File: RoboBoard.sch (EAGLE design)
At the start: 23 parts, among them IC2 L293D

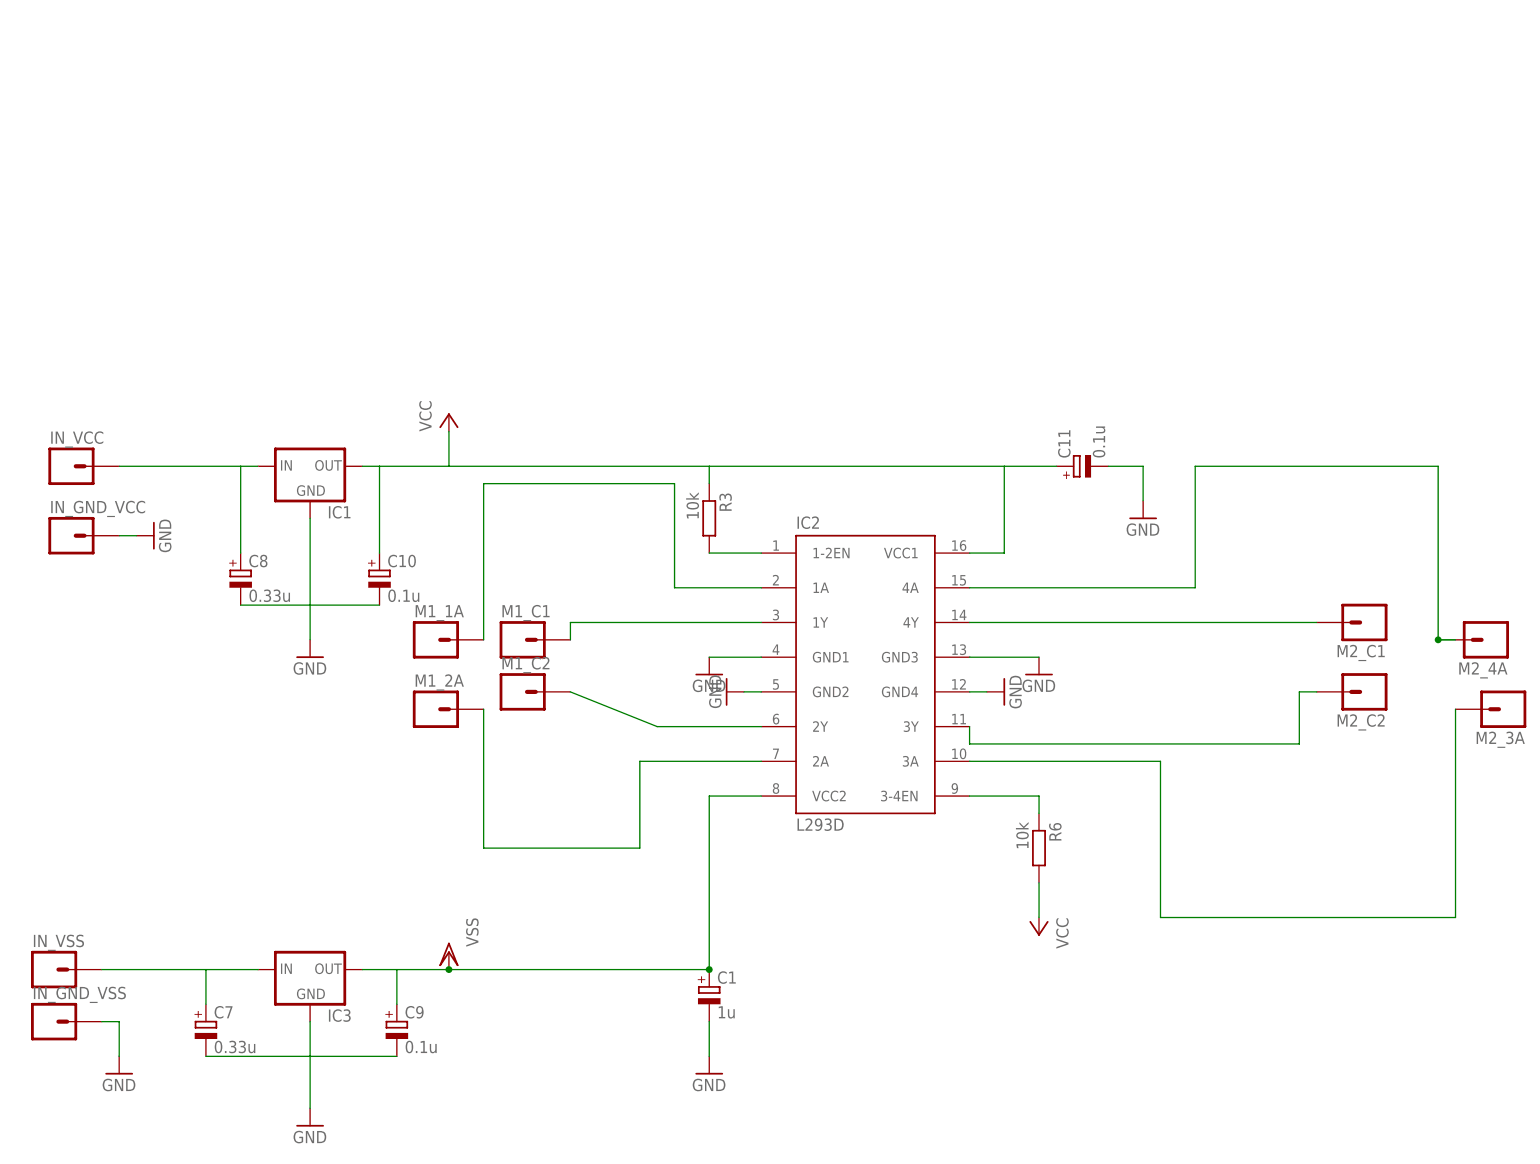
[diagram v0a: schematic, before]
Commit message: fix:	Fixing board layout
Fixing the board layout
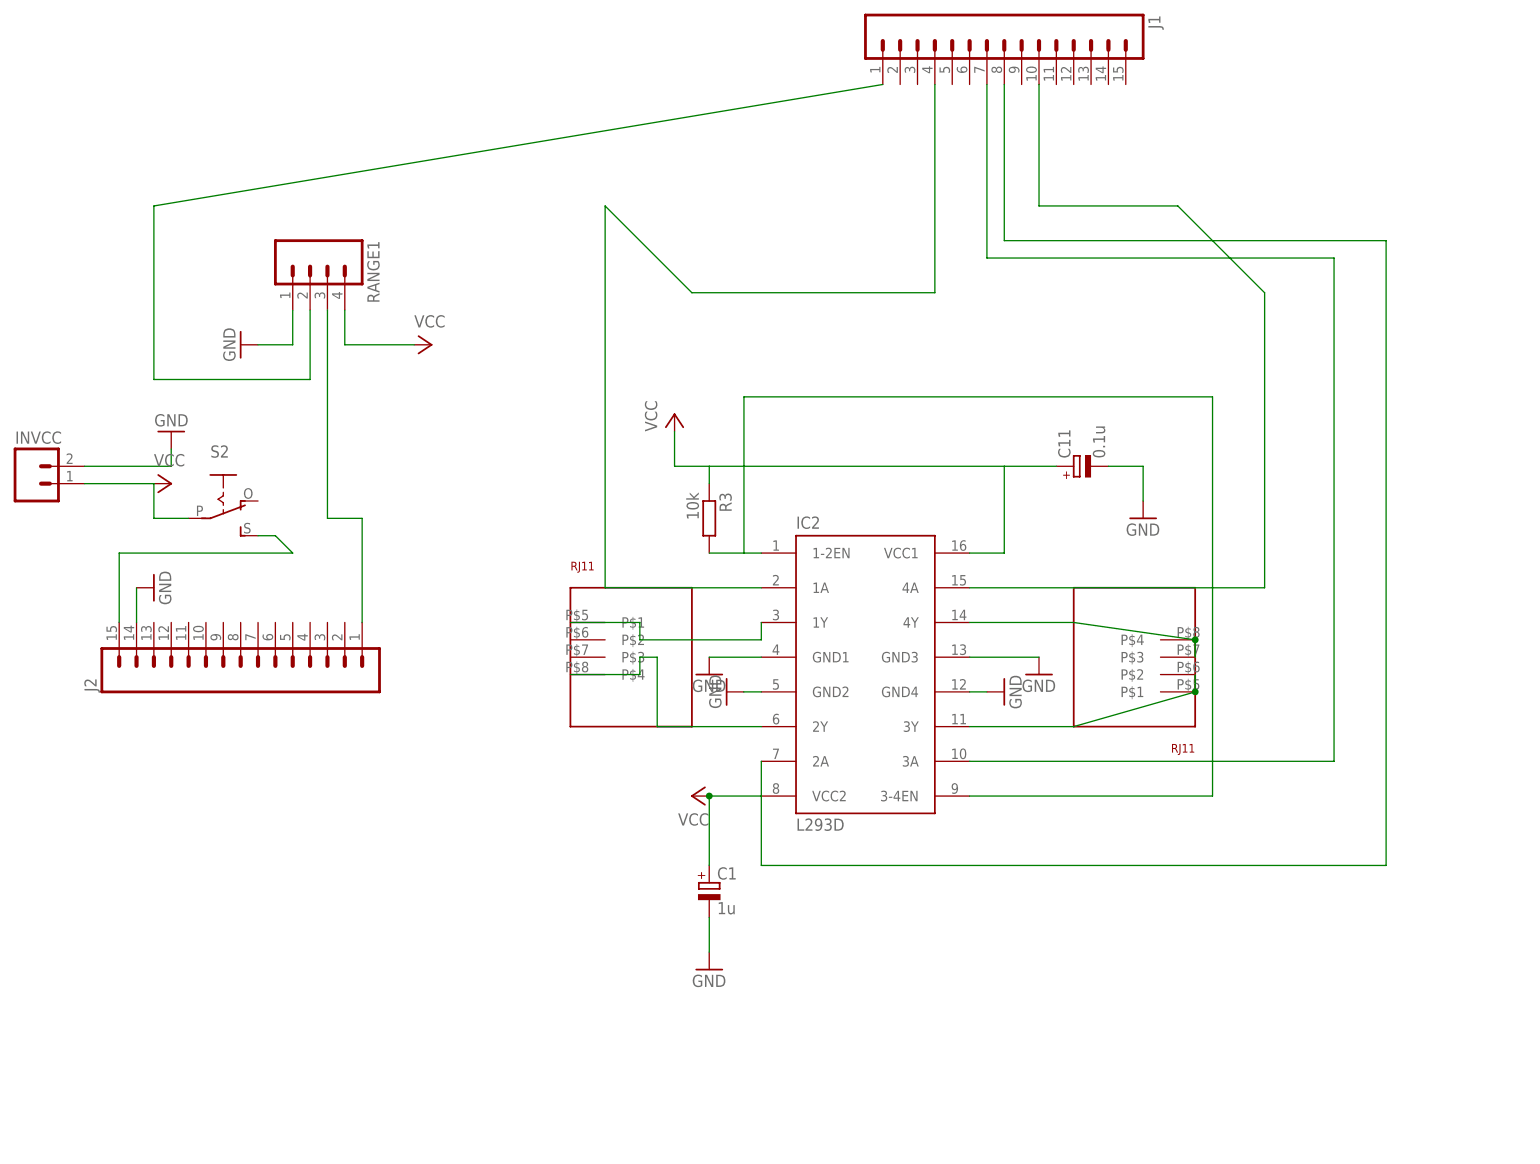
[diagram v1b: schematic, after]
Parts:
- removed C10, C9: 0.1u, resistor:CPOL-EUE1.8-4
- removed C7, C8: 0.33u, resistor:CPOL-EUE1.8-4
- removed IC1, IC3: (no value), v-reg:78XXL
- removed IN_GND_VCC, IN_GND_VSS, IN_VCC, IN_VSS, M1_1A, M1_2A, M1_C1, M1_C2, M2_3A, M2_4A, M2_C1, M2_C2: (no value), SparkFun-Connectors:M01PTH_LONGPAD
- removed R6: 10k, resistor:R-EU_0204/7
- added INVCC: (no value), SparkFun-Connectors:M02LOCK_LONGPADS
- added J1, J2: (no value), SparkFun-Connectors:M15LOCK_LONGPADS
- added RANGE1: (no value), SparkFun-Connectors:M04LONGPADS
- added RJ1, RJ2: (no value), rj11:RJ11
- added S2: (no value), adafruit:EG1218S
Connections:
- removed net N$11: IC2.1A, M1_1A.1
- removed net N$14: IC2.3A, M2_3A.1
- removed net VSS: C1.+, C9.+, IC2.VCC2, IC3.OUT
- new net N$2: IC2.2Y, RJ1.P$4
- new net N$7: IC2.3A, J1.7
- net GND: now also INVCC.2, J2.14, RANGE1.1; no longer C10.-, C7.-, C8.-, C9.-, IC1.GND, IC3.GND, IN_GND_VCC.1, IN_GND_VSS.1
- net N$1: now also IC2.1Y, RJ1.P$1; no longer IC2.1-2EN, R3.2
- net N$10: now also IC2.1A, J1.4; no longer IC2.3Y, M2_C2.1
- net N$12: now also J1.1, RANGE1.2; no longer IC2.2A, M1_2A.1
- net N$13: now also J2.15, S2.S; no longer IC2.4A, M2_4A.1
- net N$3: now also IC2.3Y, RJ2.P$1, RJ2.P$2; no longer IC2.1Y, M1_C1.1
- net N$4: now also IC2.4Y, RJ2.P$3, RJ2.P$4; no longer IC2.2Y, M1_C2.1
- net N$5: now also IC2.4A, J1.10; no longer C7.+, IC3.IN, IN_VSS.1
- net N$6: now also J2.1, RANGE1.3; no longer C8.+, IC1.IN, IN_VCC.1
- net N$8: now also IC2.1-2EN, R3.2; no longer R6.1
- net N$9: now also IC2.2A, J1.8; no longer IC2.4Y, M2_C1.1
- net VCC: now also C1.+, IC2.VCC2, INVCC.1, RANGE1.4, S2.P; no longer C10.+, IC1.OUT, R6.2
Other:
- moved on the sheet: C1
